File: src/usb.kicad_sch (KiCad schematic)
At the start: 16 parts, among them J3 USB_C_Receptacle_USB2.0_14P, J4 USB_C_Receptacle_USB2.0_14P, J5 USB_C_Receptacle_USB2.0_14P, U1 ECP5U_12_CABGA256, U5 TPD2EUSB30, U6 TPD2EUSB30, U7 FT231XQ, U8 TPD2EUSB30

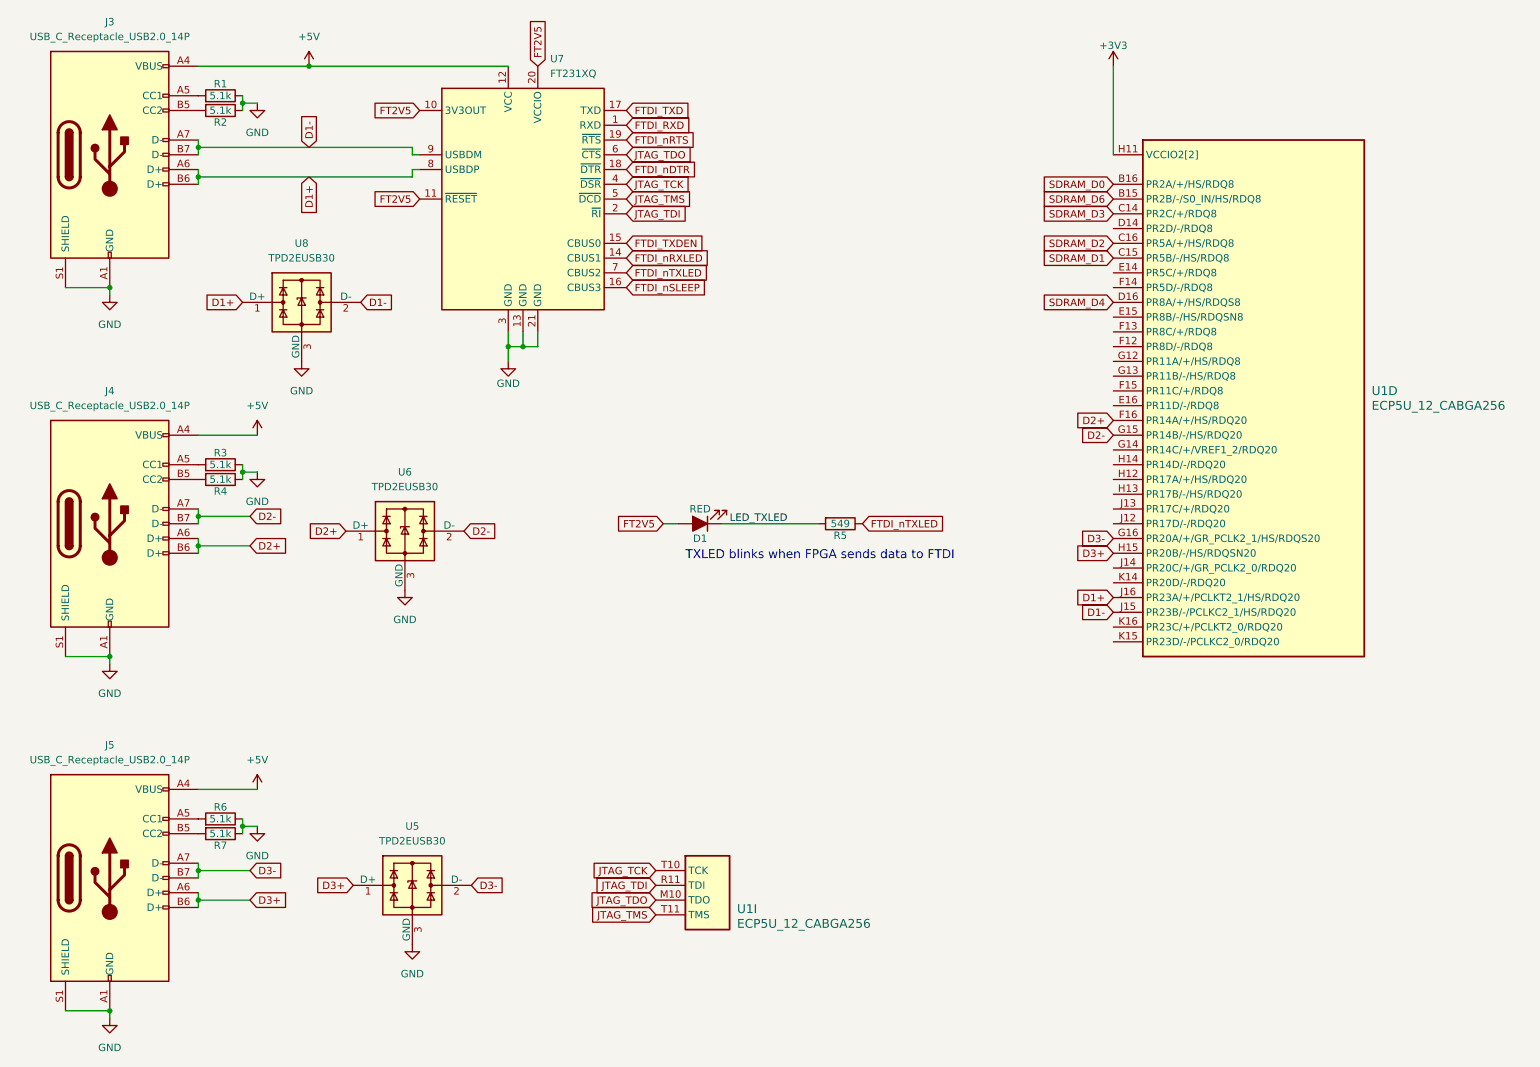
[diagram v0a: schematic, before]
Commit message: Rev 2
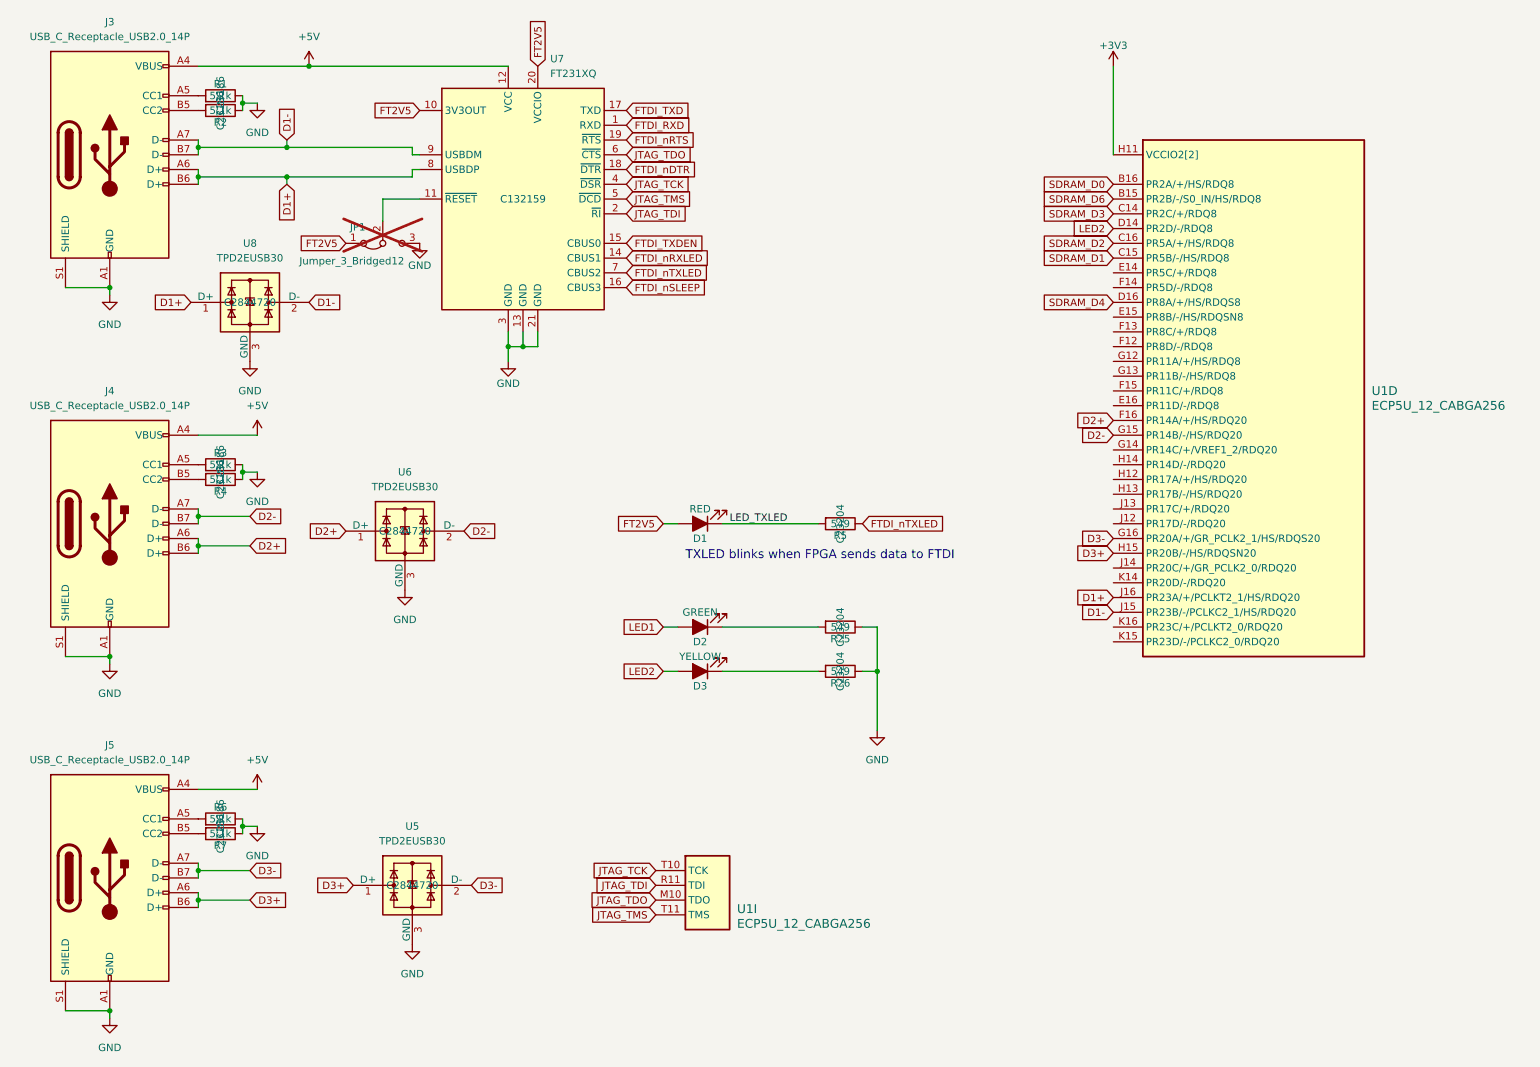
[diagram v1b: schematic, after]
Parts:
- added D2: GREEN, LED_SMD:LED_0603_1608Metric, symbol Device:LED_ALT
- added D3: YELLOW, LED_SMD:LED_0603_1608Metric, symbol Device:LED_ALT
- added JP1: Jumper_3_Bridged12, Jumper:SolderJumper-3_P1.3mm_Bridged2Bar12_RoundedPad1.0x1.5mm, symbol Jumper:Jumper_3_Bridged12
- added R25, R26: 549, Resistor_SMD:R_0603_1608Metric, symbol Device:R
- D1: LCSC Part (none) -> C2286
- R1, R2, R3, R4, R6, R7: LCSC Part (none) -> C23186
- R5: LCSC Part (none) -> C23204
- U5, U6, U8: LCSC Part (none) -> C2844720
- U7: LCSC Part (none) -> C132159
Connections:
- net FT2V5: now also JP1.1 (A); no longer U7.11 (~{RESET})
- net GND: now also JP1.3 (B), R25.1, R26.1
- net LED2: now reaches U1.D14 (PR2D/-/RDQ8)
- net LED2: now also D3.2 (A)
- new net: D3.1 (K), R26.2
- new net: JP1.2 (C), U7.11 (~{RESET})
- new net: D2.1 (K), R25.2
- new net LED1: D2.2 (A)
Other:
- moved on the sheet: U8

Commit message: Tidy project
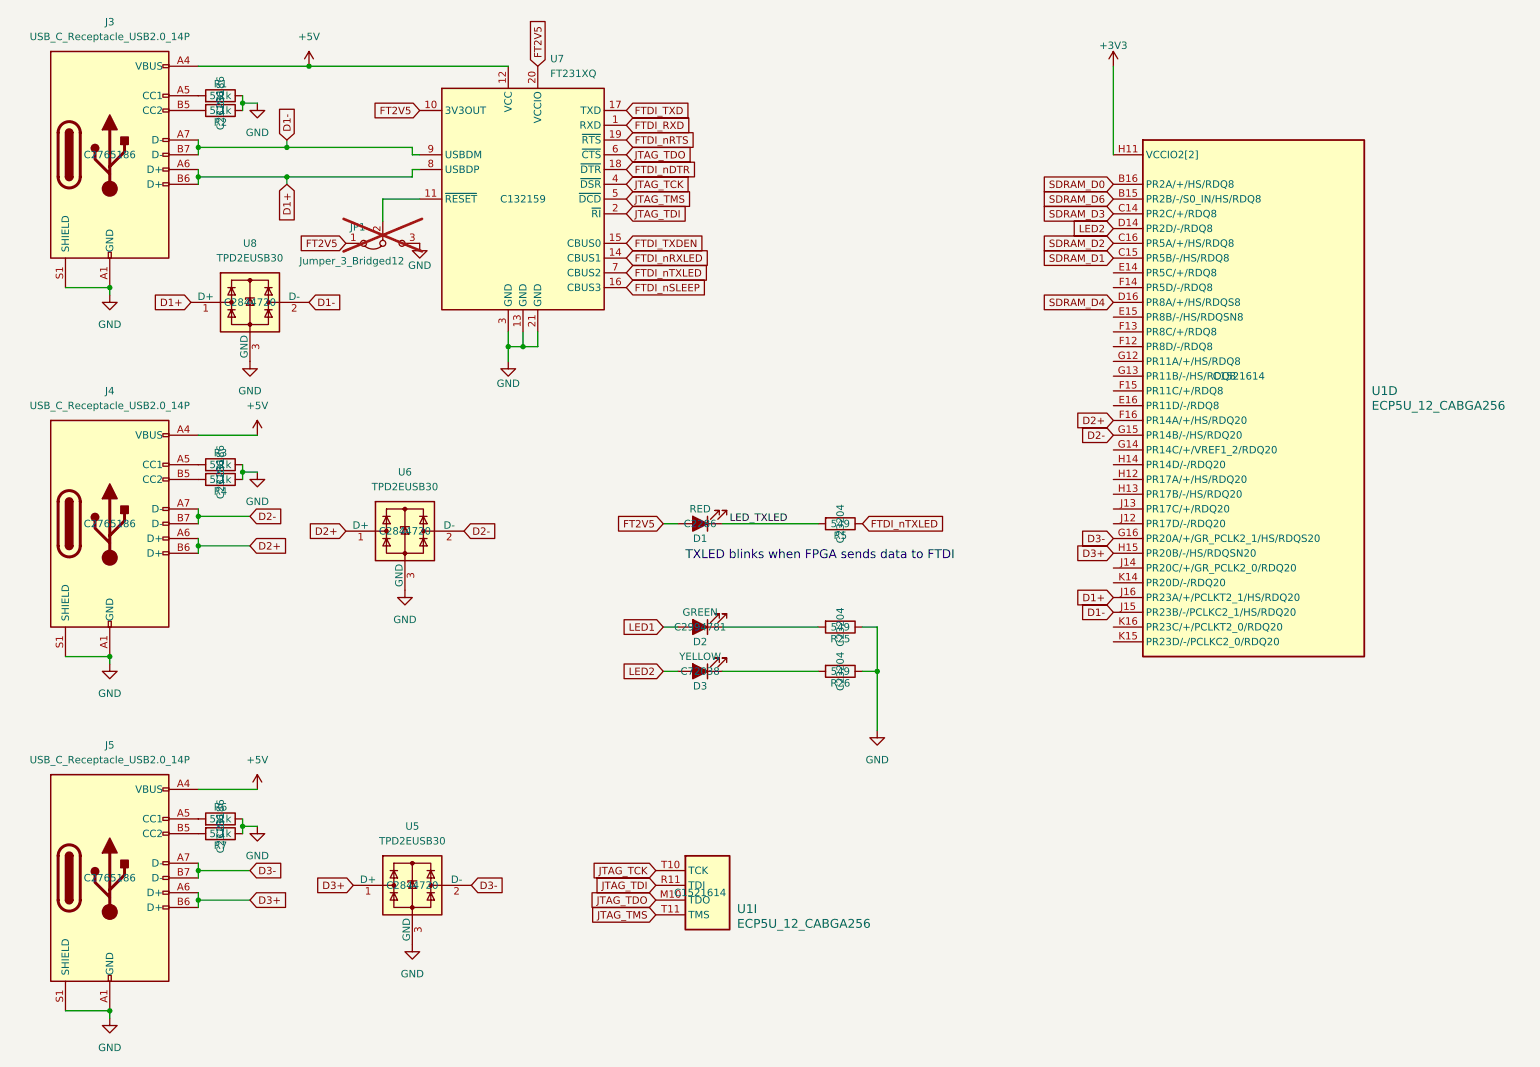
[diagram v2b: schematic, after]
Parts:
- D1: JLCPCB Part # (none) -> C2286; LCSC Part C2286 -> (none)
- D2: JLCPCB Part # (none) -> C2994781; LCSC Part C2994781 -> (none)
- D3: JLCPCB Part # (none) -> C72038; LCSC Part C72038 -> (none)
- J3, J4, J5: JLCPCB Part # (none) -> C2765186; LCSC Part C2765186 -> (none)
- R1, R2, R3, R4, R6, R7: JLCPCB Part # (none) -> C23186; LCSC Part C23186 -> (none)
- R25, R26, R5: JLCPCB Part # (none) -> C23204; LCSC Part C23204 -> (none)
- U1: JLCPCB Part # (none) -> C1521614; LCSC Part C1521614 -> (none)
- U5, U6, U8: JLCPCB Part # (none) -> C2844720; LCSC Part C2844720 -> (none)
- U7: JLCPCB Part # (none) -> C132159; LCSC Part C132159 -> (none)
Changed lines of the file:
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@@
 			)
 		)
-		(property "LCSC Part" "C2286"
+		(property "JLCPCB Part #" "C2286"
 			(at 142.24 104.14 0)
 			(effects
@@
 					(size 1.27 1.27)
 				)
-				(hide yes)
 			)
 		)
@@
 			)
 		)
-		(property "LCSC Part" "C23204"
+		(property "JLCPCB Part #" "C23204"
 			(at 166.37 104.14 0)
 			(effects
@@
 			)
 		)
-		(property "LCSC Part" "C23186"
+		(property "JLCPCB Part #" "C23186"
 			(at 59.69 96.52 0)
 			(effects
@@
 			)
 		)
-		(property "LCSC Part" "C23204"
+		(property "JLCPCB Part #" "C23204"
 			(at 166.37 129.54 0)
 			(effects
@@
 			)
 		)
-		(property "LCSC Part" " C1521614"
+		(property "JLCPCB Part #" " C1521614"
 			(at 142.24 167.64 0)
 			(effects
@@
 					(size 1.27 1.27)
 				)
-				(hide yes)
 			)
 		)
@@
 			)
 		)
-		(property "LCSC Part" "C132159"
+		(property "JLCPCB Part #" "C132159"
 			(at 111.76 48.26 0)
 			(effects
@@
 			)
 		)
-		(property "LCSC Part" "C23204"
+		(property "JLCPCB Part #" "C23204"
 			(at 166.37 121.92 0)
 			(effects
@@
 			)
 		)
-		(property "LCSC Part" "C23186"
+		(property "JLCPCB Part #" "C23186"
 			(at 59.69 33.02 0)
 			(effects
@@
 			)
 		)
-		(property "LCSC Part" "C23186"
+		(property "JLCPCB Part #" "C23186"
 			(at 59.69 93.98 0)
 			(effects
@@
 			)
 		)
-		(property "LCSC Part" "C23186"
+		(property "JLCPCB Part #" "C23186"
 			(at 59.69 30.48 0)
 			(effects
@@
 			)
 		)
-		(property "LCSC Part" "C72038"
+		(property "JLCPCB Part #" "C72038"
 			(at 142.24 129.54 0)
 			(effects
@@
 					(size 1.27 1.27)
 				)
-				(hide yes)
 			)
 		)
@@
 			)
 		)
-		(property "LCSC Part" "C2844720"
+		(property "JLCPCB Part #" "C2844720"
 			(at 91.44 105.41 0)
 			(effects
@@
 			)
 		)
-		(property "LCSC Part" "C23186"
+		(property "JLCPCB Part #" "C23186"
 			(at 59.69 157.48 0)
 			(effects
@@
 			)
 		)
-		(property "LCSC Part" " C2765186"
+		(property "JLCPCB Part #" " C2765186"
 			(at 40.64 40.64 0)
 			(effects
@@
 					(size 1.27 1.27)
 				)
-				(hide yes)
 			)
 		)
@@
 			)
 		)
-		(property "LCSC Part" ""
-			(at 87.63 55.88 0)
-			(effects
-				(font
-					(size 1.27 1.27)
-				)
-				(hide yes)
-			)
-		)
 		(pin "3"
 		)
@@
 			)
 		)
-		(property "LCSC Part" "C23186"
+		(property "JLCPCB Part #" "C23186"
 			(at 59.69 154.94 0)
 			(effects
@@
 			)
 		)
-		(property "LCSC Part" " C2765186"
+		(property "JLCPCB Part #" " C2765186"
 			(at 40.64 165.1 0)
 			(effects
@@
 					(size 1.27 1.27)
 				)
-				(hide yes)
 			)
 		)
@@
 			)
 		)
-		(property "LCSC Part" "C2844720"
+		(property "JLCPCB Part #" "C2844720"
 			(at 64.77 66.04 0)
 			(effects
@@
 			)
 		)
-		(property "LCSC Part" "C2994781"
+		(property "JLCPCB Part #" "C2994781"
 			(at 142.24 121.92 0)
 			(effects
@@
 					(size 1.27 1.27)
 				)
-				(hide yes)
 			)
 		)
@@
 			)
 		)
-		(property "LCSC Part" " C1521614"
+		(property "JLCPCB Part #" " C1521614"
 			(at 234.95 78.74 0)
 			(effects
@@
 					(size 1.27 1.27)
 				)
-				(hide yes)
 			)
 		)
@@
 			)
 		)
-		(property "LCSC Part" "C2844720"
+		(property "JLCPCB Part #" "C2844720"
 			(at 92.71 166.37 0)
 			(effects
@@
 			)
 		)
-		(property "LCSC Part" " C2765186"
+		(property "JLCPCB Part #" " C2765186"
 			(at 40.64 104.14 0)
 			(effects
@@
 					(size 1.27 1.27)
 				)
-				(hide yes)
 			)
 		)
